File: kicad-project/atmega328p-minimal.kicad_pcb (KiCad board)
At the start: 2 copper layers, 22.9 x 48.3 mm, 9 parts, among them IC1 ATMEGA328-P, P1 CONN_01X02, P2 CONN_01X16, P3 CONN_01X16, SW1 SW_PUSH, Y1 16MHz

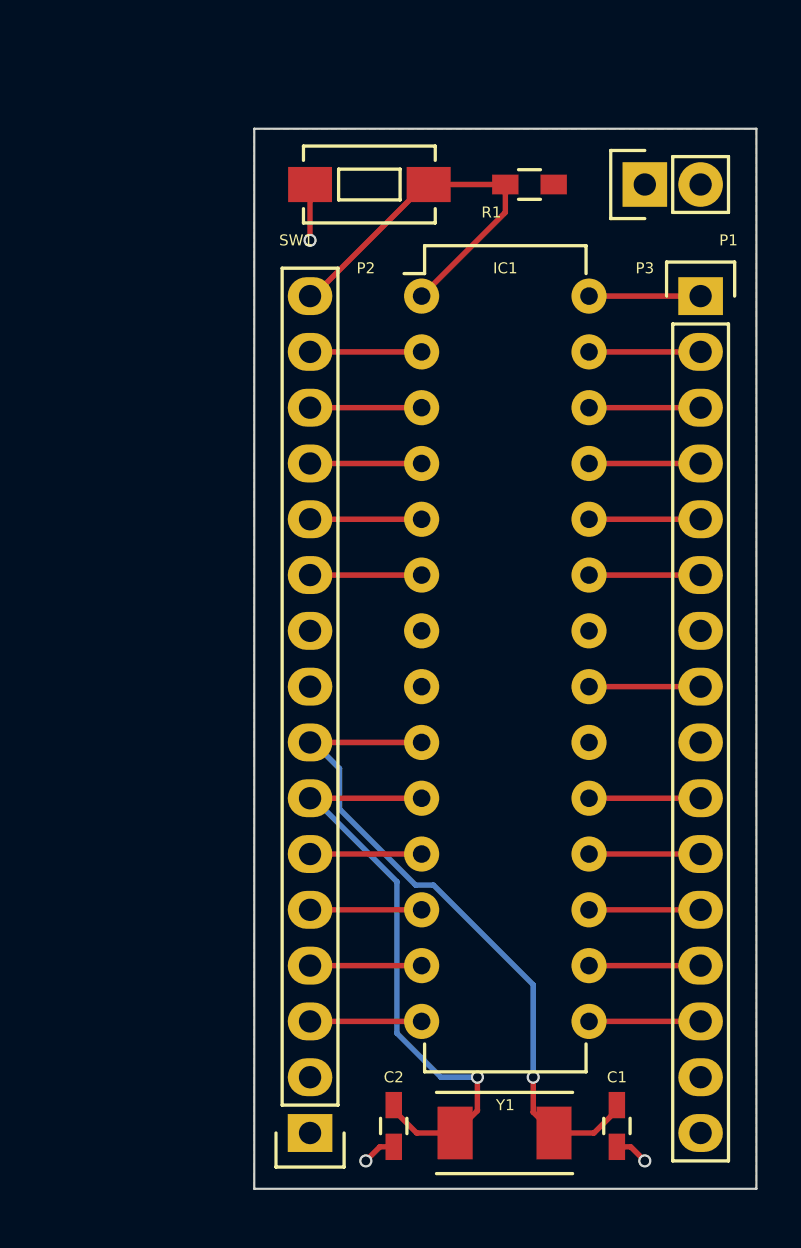
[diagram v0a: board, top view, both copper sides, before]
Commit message: Changed KiCad project, schematics and board design for this version.
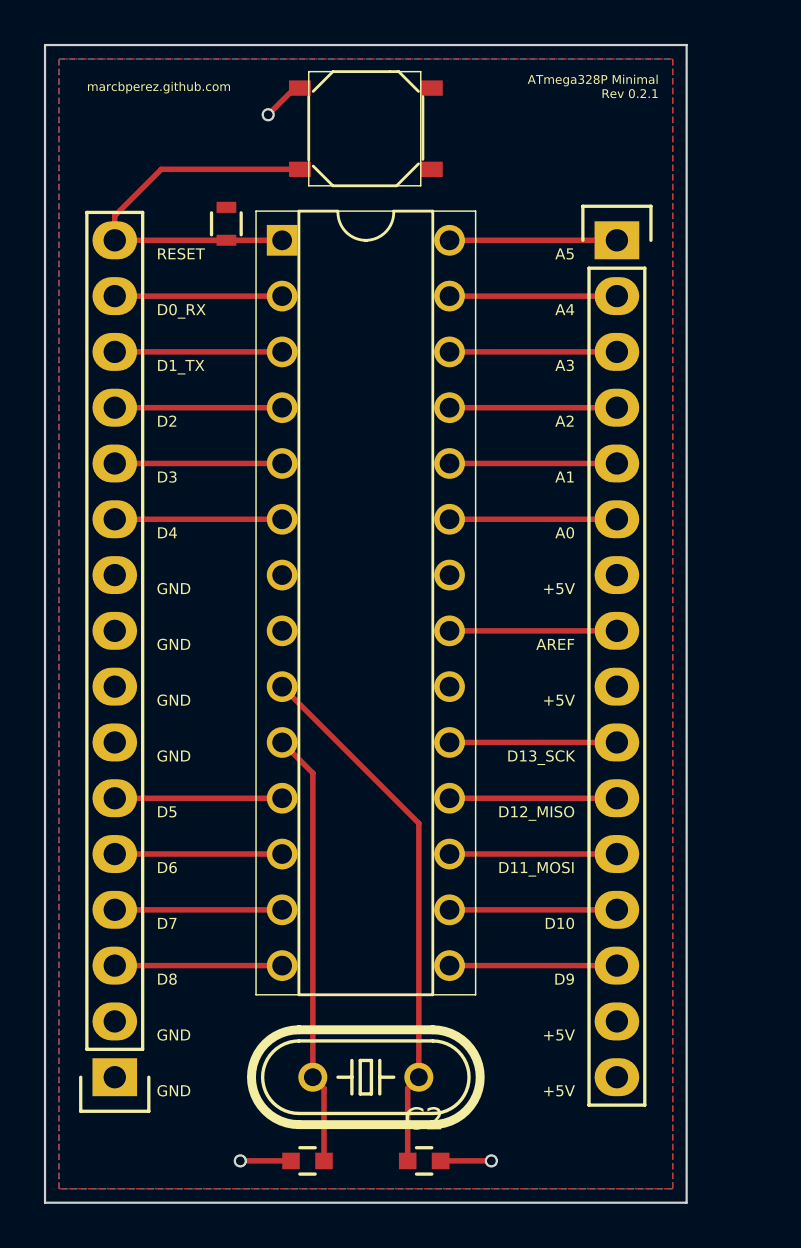
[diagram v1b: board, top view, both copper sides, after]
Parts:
- removed IC1: ATMEGA328-P, Housings_DIP:DIP-28_W7.62mm
- removed P1: CONN_01X02, Pin_Headers:Pin_Header_Straight_1x02
- added U1: MCU-ATMEGA328P-PU_DIP28_, SeeedOPL-IC-2016:DIP28-2.54-34.7X7.62MM, F.Cu at (146.1, 100.3)
- C1, C2: footprint Capacitors_SMD:C_0603_HandSoldering -> Capacitors_SMD:C_0603
- R1: footprint Resistors_SMD:R_0603_HandSoldering -> Resistors_SMD:R_0603
- SW1: value SW_PUSH -> SMD-BUTTON_4P-5.2X5.2X1.5MM-SKQGADE010_; footprint Buttons_Switches_SMD:SW_SPST_EVQPE1 -> SeeedOPL-Switch-2016:SW4-SMD-5.2X5.2X1.5MM
- Y1: value 16MHz -> DIP-CRYSTAL-16MHZ-18PF-30PPM-40R_HC49US_; footprint Crystals:Crystal_SMD_0603_2Pads_obsolete -> SeeedOPL-Crystal Oscillator-2016:HC49US
- moved C1 14.2 mm to (143.4, 125.7), turned to 180 degrees
- moved R1 13.9 mm to (139.7, 83.1), turned to 270 degrees
- moved P2 9.25 mm to (134.6, 121.9)
- moved Y1 6.81 mm to (146.1, 121.9)
- moved P3 4.58 mm to (157.5, 83.8)
- moved SW1 2.55 mm to (146.1, 78.7)
- moved C2 2.11 mm to (148.7, 125.7), turned to 0 degrees
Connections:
- C1 pad 1: GND -> Net-(C1-Pad1)
- C1 pad 2: /XTAL1 -> GND
- C2 pad 1: GND -> Net-(C2-Pad1)
- C2 pad 2: /XTAL2 -> GND
- P2 pad 1: +5V -> GND
- P2 pad 10: +5V -> GND
- P2 pad 2: +5V -> GND
- P2 pad 7: /XTAL2 -> GND
- P2 pad 8: /XTAL1 -> GND
- P2 pad 9: +5V -> GND
- P3 pad 10: /D13 -> /D13_SCK
- P3 pad 11: /D12 -> /D12_MISO
- P3 pad 12: /D11 -> /D11_MOSI
- P3 pad 15: GND -> +5V
- P3 pad 16: GND -> +5V
- P3 pad 7: GND -> +5V
- P3 pad 9: GND -> +5V
- SW1 pad 1: /RESET -> (no net)
- SW1 pad 2: GND -> /RESET
- Y1 pad 1: /XTAL2 -> Net-(C1-Pad1)
- Y1 pad 2: /XTAL1 -> Net-(C2-Pad1)
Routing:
- net /XTAL1: track 31.6 -> 0.00 mm, vias 1 -> 0
- net /XTAL2: track 28.4 -> 0.00 mm, vias 1 -> 0
- net Net-(C2-Pad1): track 0.00 -> 24.4 mm
- net Net-(C1-Pad1): track 0.00 -> 19.8 mm
- net /D13_SCK: track 0.00 -> 7.62 mm
- net /D12_MISO: track 0.00 -> 7.62 mm
- net /D11_MOSI: track 0.00 -> 7.62 mm
- net /D13: track 5.08 -> 0.00 mm
- net /D12: track 5.08 -> 0.00 mm
- net /D11: track 5.08 -> 0.00 mm
- net /D9: track 5.08 -> 7.62 mm
- net /D8: track 5.08 -> 7.62 mm
- net /D7: track 5.08 -> 7.62 mm
- net /D6: track 5.08 -> 7.62 mm
- net /D5: track 5.08 -> 7.62 mm
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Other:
- board size 22.9 x 48.3 mm -> 29.2 x 52.7 mm
- board text added: "+5V"
- board text added: "A0"
- board text added: "A1"
- board text added: "A2"
- board text added: "A3"
- board text added: "A4"
- board text added: "A5"
- board text added: "AREF"
- board text added: "ATmega328P Minimal Rev 0.2.1"
- board text added: "D0_RX"
- board text added: "D10"
- board text added: "D11_MOSI"
- board text added: "D12_MISO"
- board text added: "D13_SCK"
- board text added: "D1_TX"
- board text added: "D2"
- board text added: "D3"
- board text added: "D4"
- board text added: "D5"
- board text added: "D6"
- board text added: "D7"
- board text added: "D8"
- board text added: "D9"
- board text added: "GND"
- board text added: "RESET"
- board text added: "marcbperez.github.com"
